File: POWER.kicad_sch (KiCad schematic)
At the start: 22 parts, among them J100 VCC INPUT, J101 SWITCH ON/OFF, J103 FAN VOLTAGE, Q100 WST4045, U100 LM2596S-5, U101 AMS1117-3.3

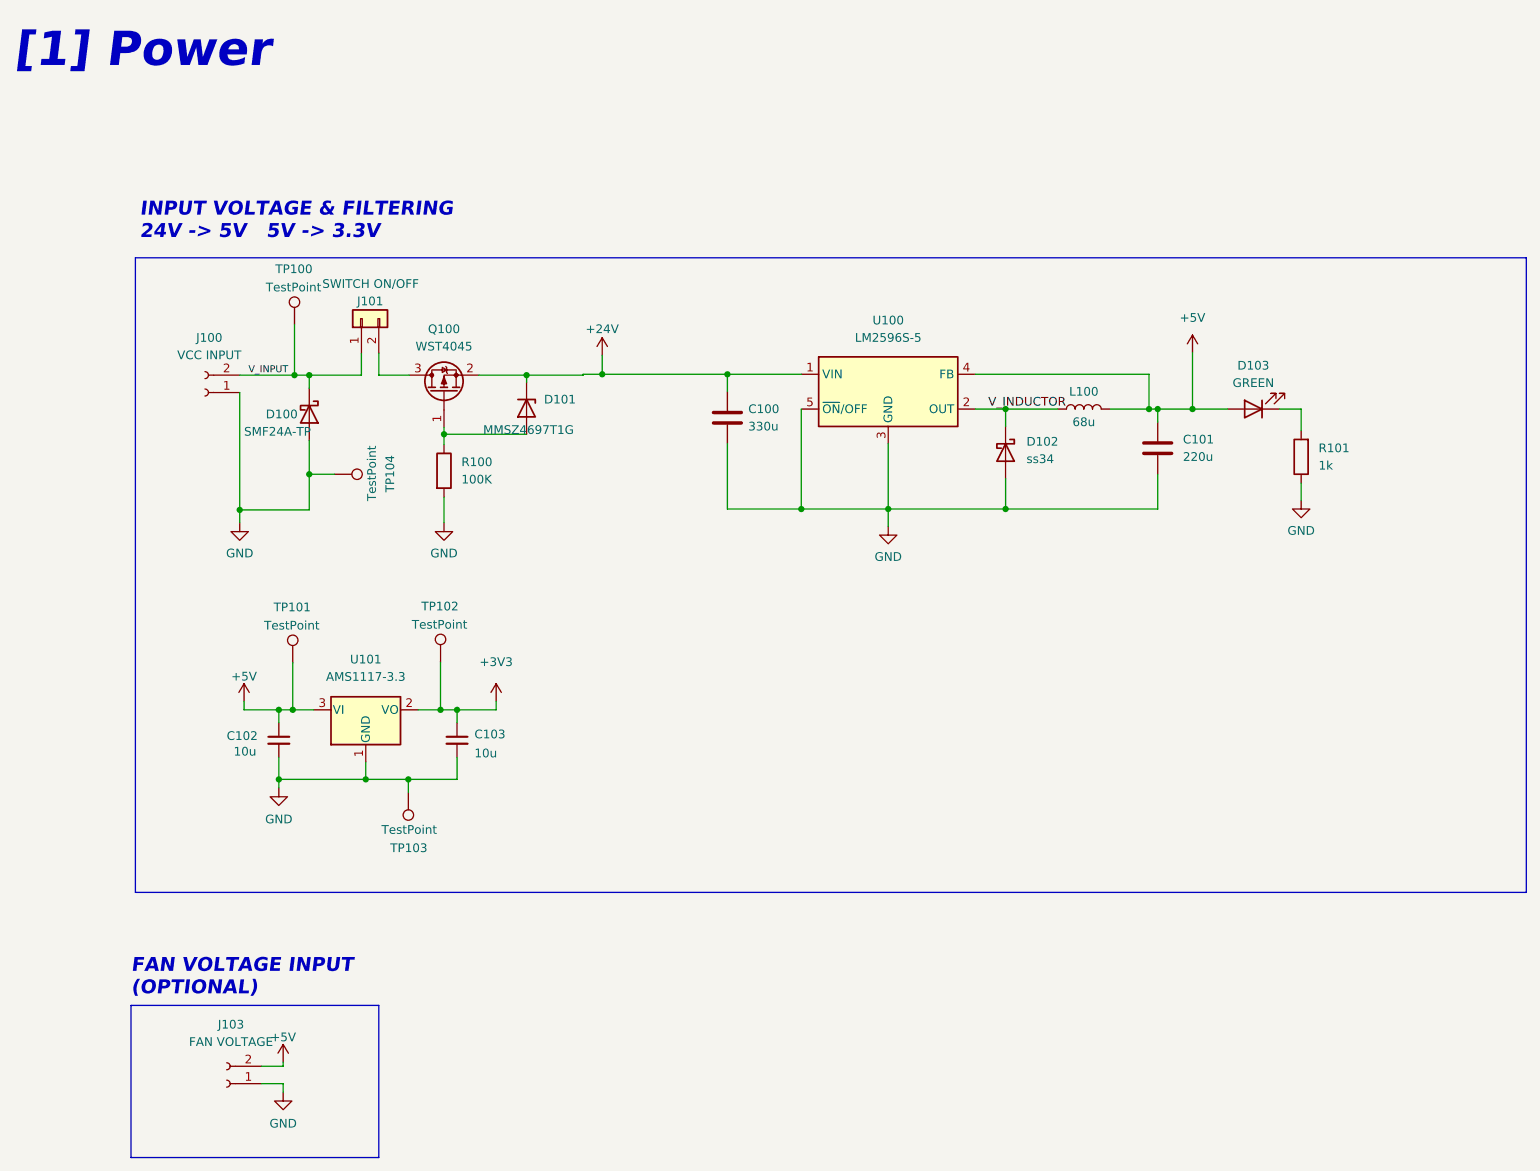
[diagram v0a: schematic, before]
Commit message: version validada
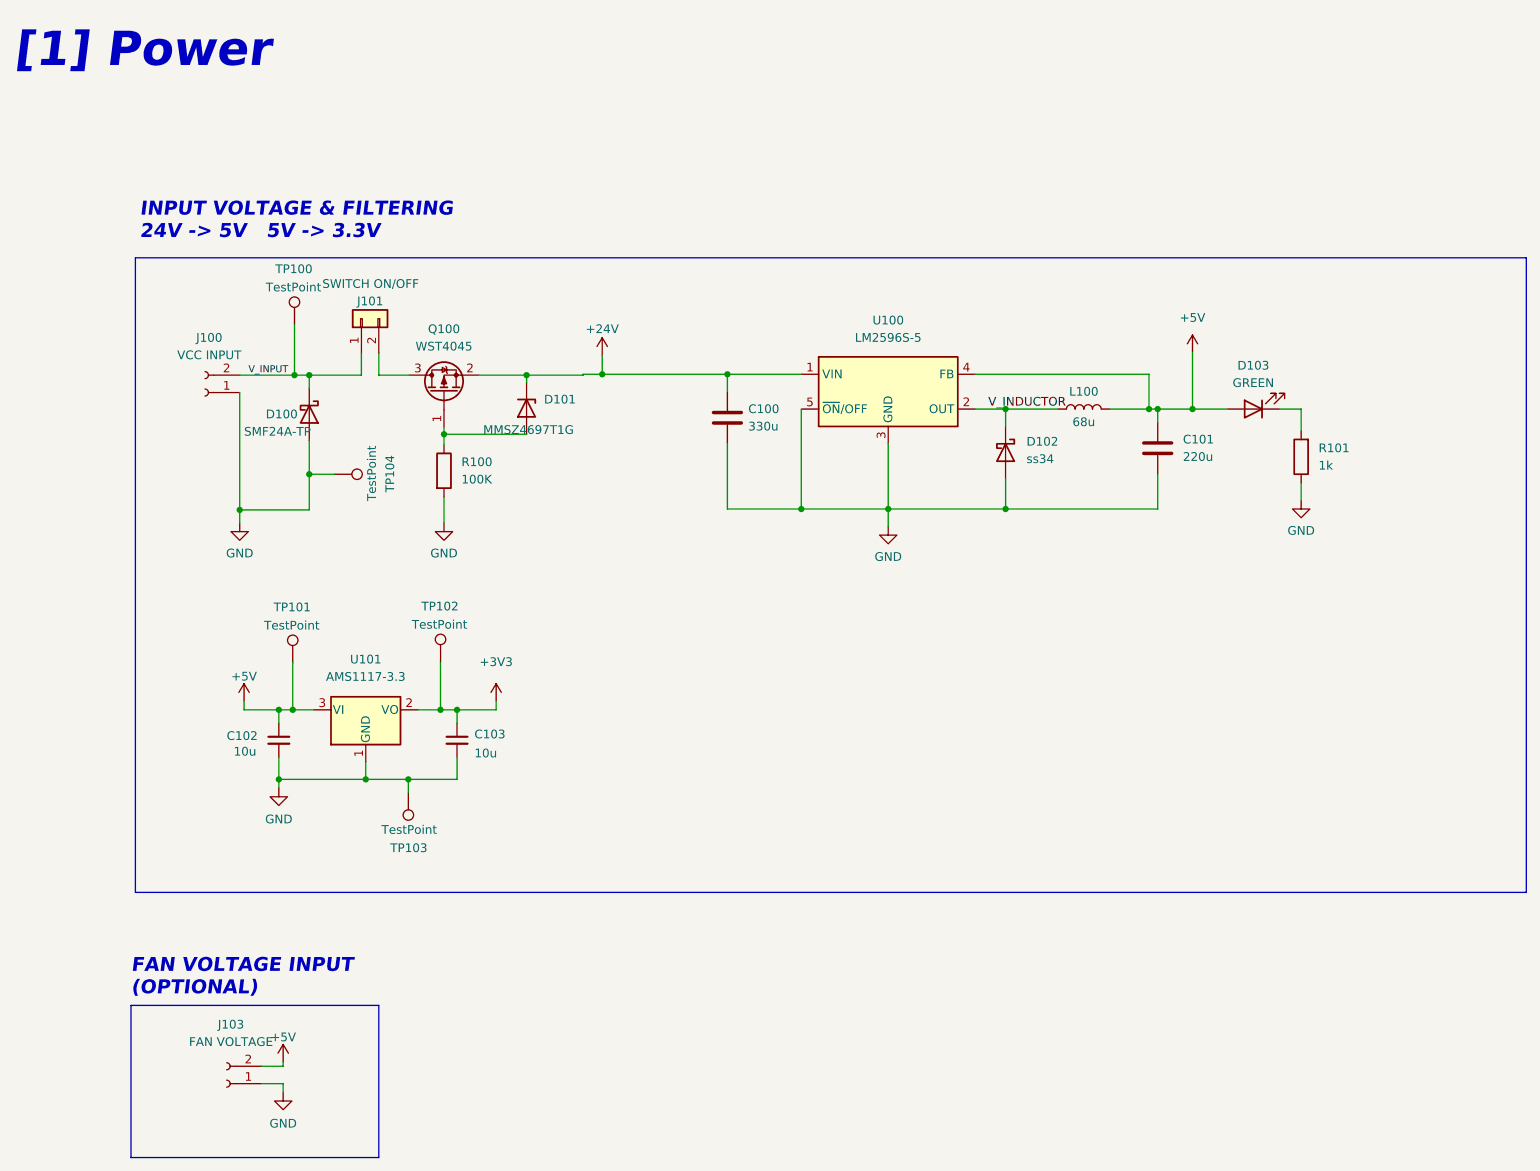
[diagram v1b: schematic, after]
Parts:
- J101: footprint Connector_PinHeader_2.54mm:PinHeader_1x02_P2.54mm_Vertical -> B2B-XH-A:JST_B2B-XH-A_LF__SN_
